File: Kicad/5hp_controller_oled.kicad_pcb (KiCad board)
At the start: 4 copper layers, 25 x 105 mm, 14 parts, among them J1 SSD1306, J2 AS5600_2_PWR, J4 AS5600_2_PWR, J5 AS5600_2_PWR

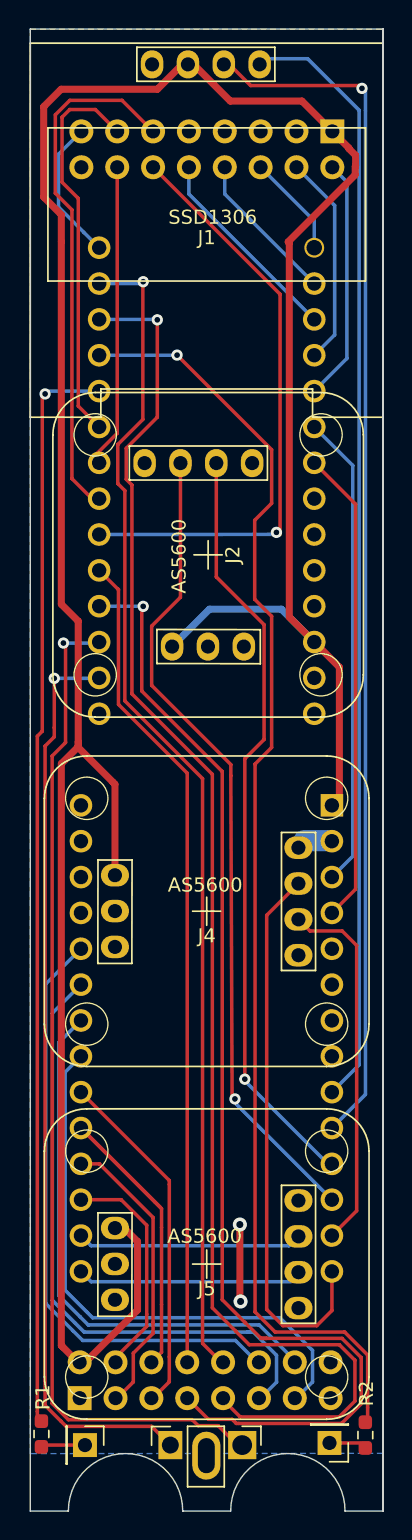
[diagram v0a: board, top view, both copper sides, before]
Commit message: Final pcb and frontpanel
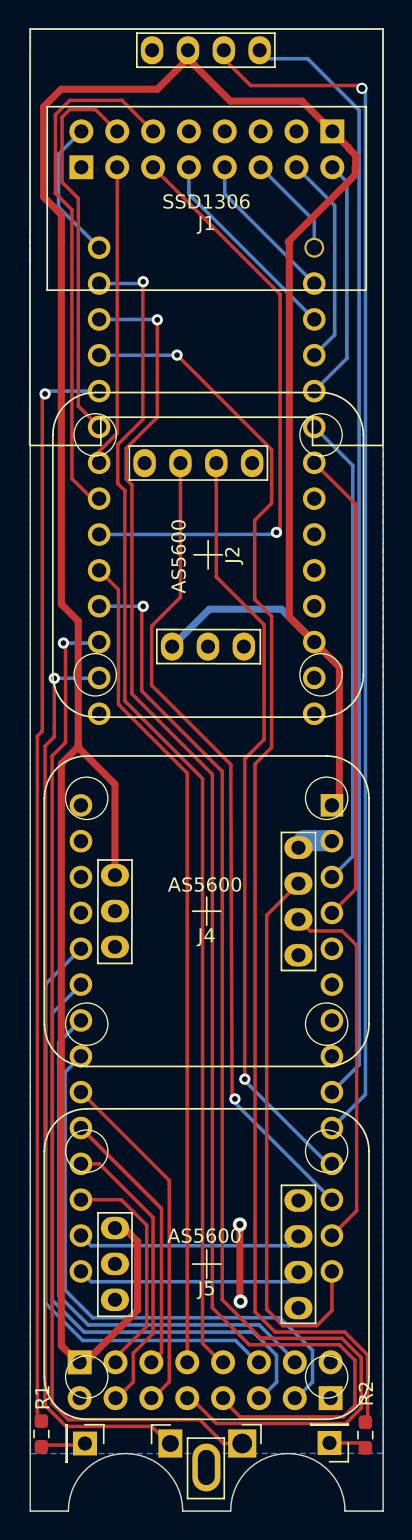
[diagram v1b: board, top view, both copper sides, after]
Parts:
- moved J1 1.00 mm to (25.0, -41.8)
- moved BTN1 0.11 mm to (22.4, 45.2)
- moved BTN2 0.11 mm to (27.5, 45.2)
- moved LED1 0.11 mm to (16.4, 45.2)
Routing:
- net BTN2: track 71.9 -> 72.6 mm
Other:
- copper layers 4 -> 2
- board text added: "+3.3V"
